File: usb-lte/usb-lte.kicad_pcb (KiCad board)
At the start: 4 copper layers, 26 x 45 mm, 64 parts, among them J1 Sim slot, J2 Conn_Coaxial, J3 Conn_Coaxial, J4 Conn_Coaxial, P1 USB_C_Plug_USB2.0, Q1 BC847W, Q2 BC847W, U1 TPS62A02APDDC, U2 EG95

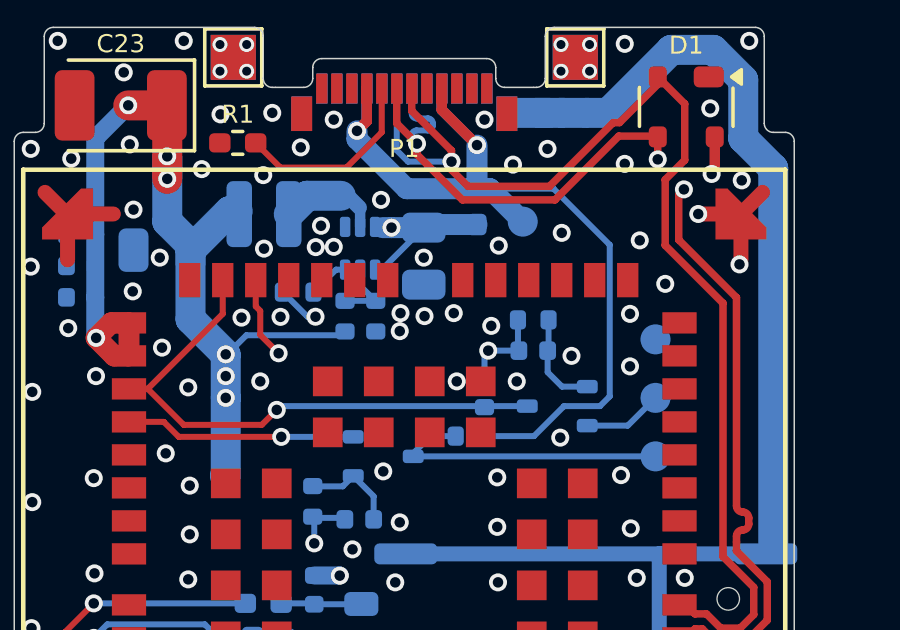
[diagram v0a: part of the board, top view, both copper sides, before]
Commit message: Minor changes
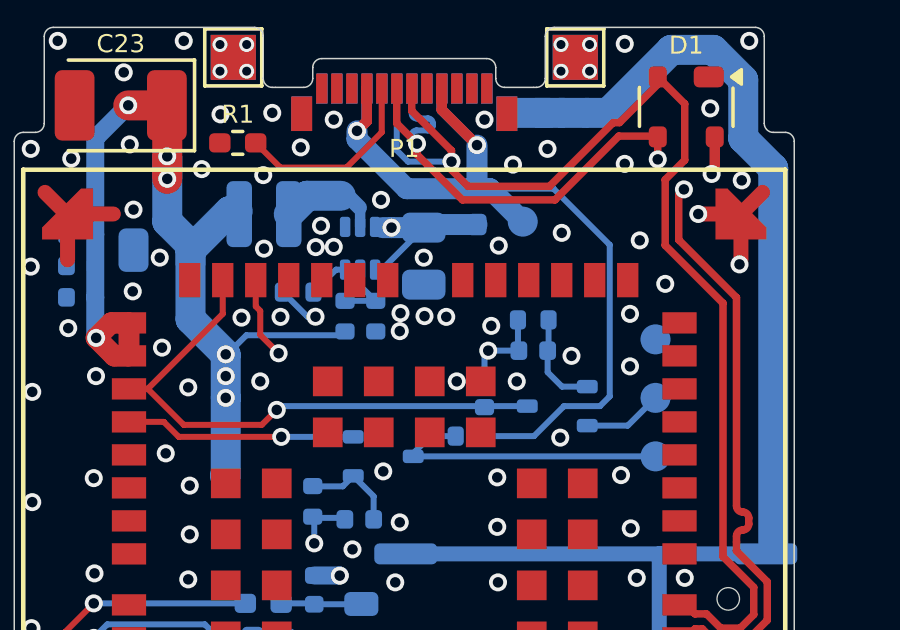
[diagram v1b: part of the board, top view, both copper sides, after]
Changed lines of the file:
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@@
 		(tags "resistor")
 		(property "Reference" "R12"
-			(at 0 1.8 0)
+			(at 1.8 0 0)
 			(layer "B.SilkS")
 			(effects
@@
 		(tags "capacitor")
 		(property "Reference" "C15"
-			(at 0 1.95 0)
+			(at 1.8 0 0)
 			(layer "B.SilkS")
 			(effects
@@
 		(tags "capacitor")
 		(property "Reference" "C1"
-			(at 0.25 -1.45 90)
+			(at -2.3 0 90)
 			(layer "B.SilkS")
 			(effects
@@
 		(tags "resistor handsolder")
 		(property "Reference" "R8"
-			(at -0.65 0.925 90)
+			(at 1.675 0 90)
 			(layer "B.SilkS")
 			(effects
@@
 	)
 	(gr_text "5V"
-		(at 156.45 95.75 0)
+		(at 155.15 96.9 0)
 		(layer "B.SilkS")
 		(effects
@@
 	)
 	(via
-		(at 152.25 98.425)
+		(at 152 98.55)
 		(size 0.6)
 		(drill 0.35)
